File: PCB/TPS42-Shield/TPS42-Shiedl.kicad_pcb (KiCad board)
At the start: 2 copper layers, 36.9 x 43.8 mm, 33 parts, among them J1 PJ-320A, J10 FH12-10S-0.5SH, J11 Conn_01x06, J12 Conn_01x01, J2 Conn_01x06, J3 OLED, J4 PJ-320A, J5 Conn_01x06, J6 OLED, J7 FH12-10S-0.5SH, J8 Conn_01x06, J9 Conn_01x01

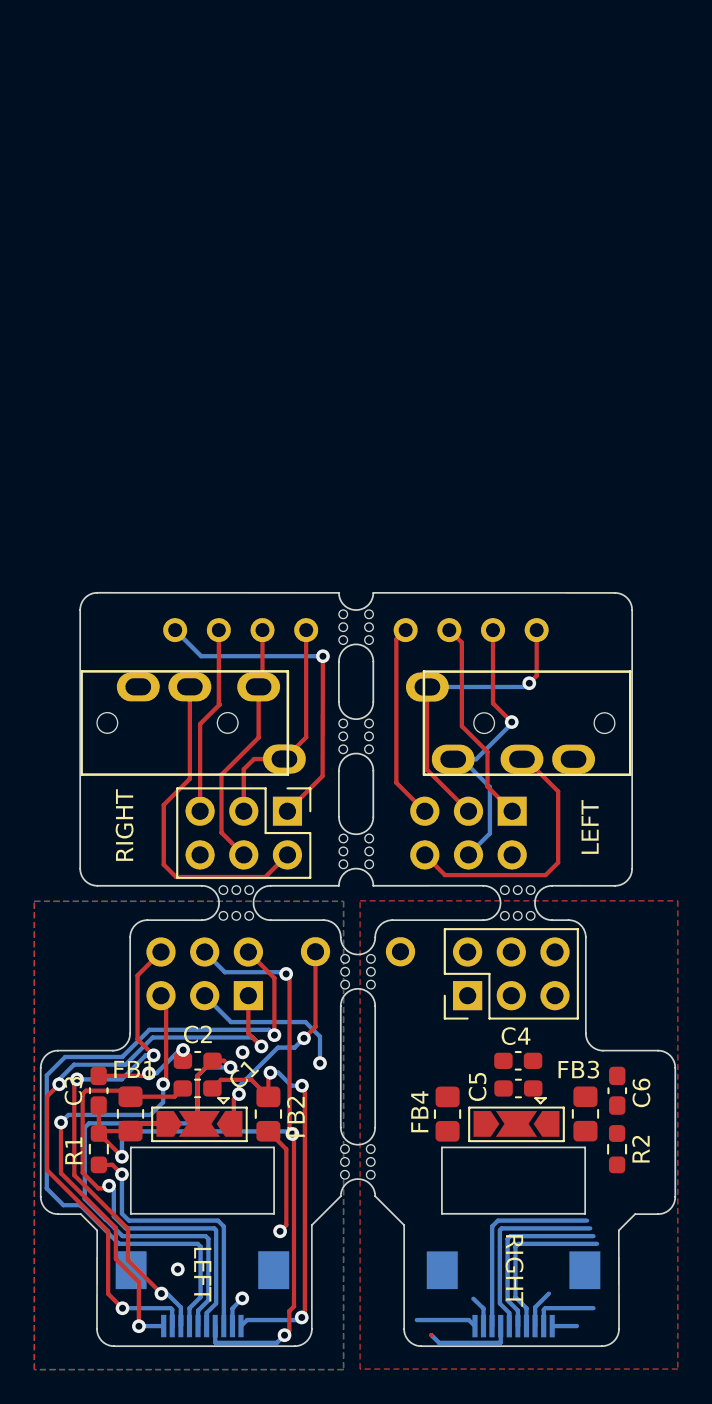
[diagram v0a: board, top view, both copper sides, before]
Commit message: finish routing
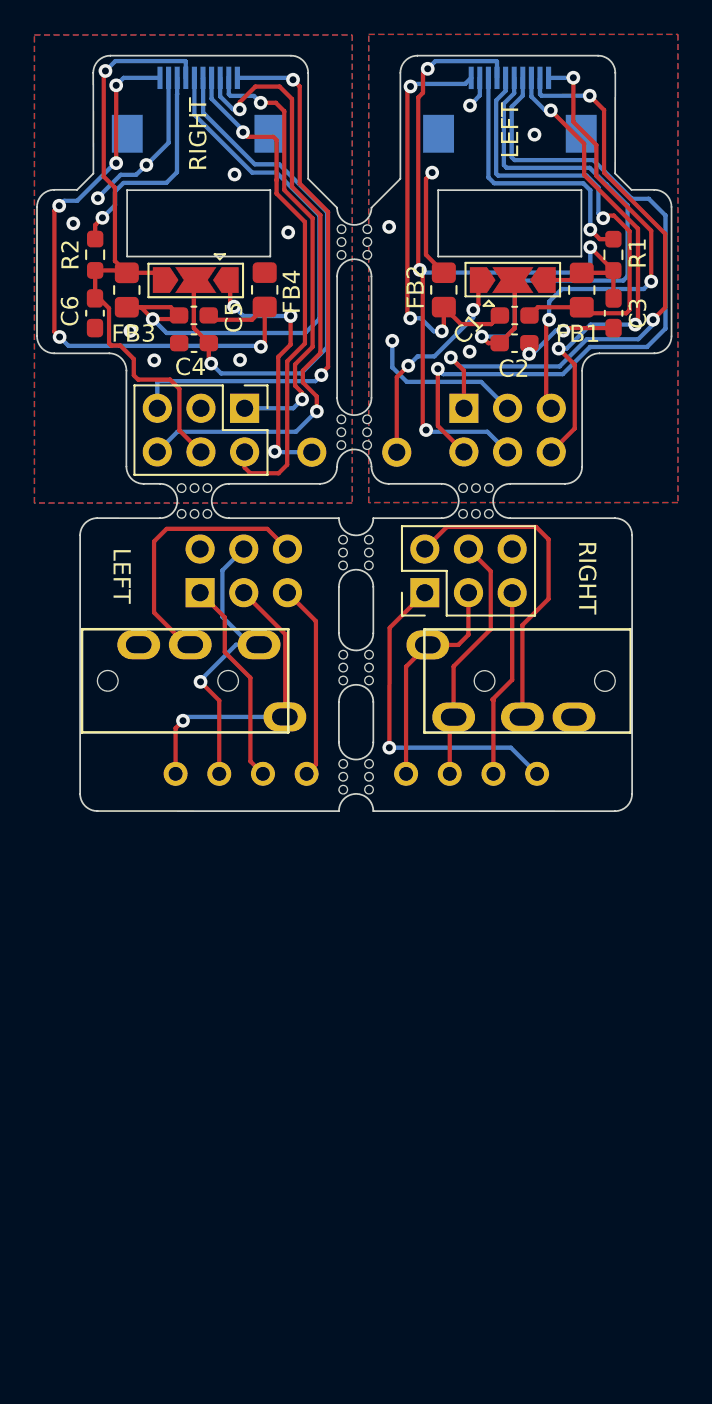
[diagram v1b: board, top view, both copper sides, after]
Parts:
- moved J10 71.3 mm to (36.4, 24.7), turned to 180 degrees
- moved J7 71.2 mm to (54.5, 24.7), turned to 180 degrees
- moved R2 60.2 mm to (30.4, 33.2), turned to 90 degrees
- moved R1 60.0 mm to (60.5, 33.2), turned to 90 degrees
- moved FB3 54.8 mm to (32.2, 35.2), turned to 90 degrees
- moved FB1 54.6 mm to (58.7, 35.2), turned to 90 degrees
- moved C6 54.5 mm to (30.4, 36.6), turned to -90 degrees
- moved C3 54.2 mm to (60.5, 36.6), turned to -90 degrees
- moved mouse-bite-2mm-slot 53.5 mm to (45.5, 32.4), turned to 90 degrees
- moved JP2 52.5 mm to (36.2, 34.6)
- moved JP1 52.4 mm to (54.7, 34.7), turned to 0 degrees
- moved FB4 49.1 mm to (40.2, 35.2), turned to 90 degrees
- moved FB2 49.0 mm to (50.7, 35.2), turned to 90 degrees
- moved C5 48.8 mm to (36.1, 36.7), turned to 0 degrees
- moved C2 48.6 mm to (54.8, 36.7), turned to 180 degrees
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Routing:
- net GNDA: track 26.3 -> 62.3 mm, vias 3 -> 8
- net /R_CLK: track 3.94 -> 32.7 mm, vias 0 -> 2
- net +3V3: track 60.8 -> 87.8 mm, vias 4 -> 5
- net /R_CS: track 11.5 -> 36.5 mm, vias 0 -> 2
- net /R_EIN: track 5.19 -> 29.9 mm, vias 0 -> 1
- net VDDA: track 37.2 -> 61.6 mm, vias 1 -> 2
- net /R_DAT: track 1.84 -> 26.2 mm, vias 0 -> 2
- net /R_DISP: track 11.7 -> 32.4 mm, vias 0 -> 1
- net Net-(J12-Pad1): track 0.00 -> 15.6 mm, vias 0 -> 3
- net /R_EXTMODE: track 2.22 -> 12.8 mm, vias 0 -> 1
- net GND: track 26.9 -> 32.2 mm, vias 7 -> 16
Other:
- board size 36.9 x 43.8 mm -> 36.9 x 43.9 mm
